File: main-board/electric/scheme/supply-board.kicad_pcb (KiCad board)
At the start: 2 copper layers, 74 x 56 mm, 136 parts, among them K1 CONN_3, P1 PWR-IN, P10 TST, P11 TST, P12 PWR-IN, P13 CONN_4, P14 PWR-IN, P16 TST, P2 PWR-IN, P3 CONN_4, P4 cross board conn, P5 PWR-IN, P6 TST, P7 TST, P8 TST, P9 CONN_3X2, Q1 BC847, Q10 MOS_N, Q11 MOS_P, Q12 MOS_P, Q2 BC847, Q3 BC847, Q4 MOS_P, Q5 BC847, Q6 BC857, Q7 BC847, Q8 BC857, Q9 BC847, U1 NCP3063, U2 L293, U3 MINI-USB-B, X1 8MHz

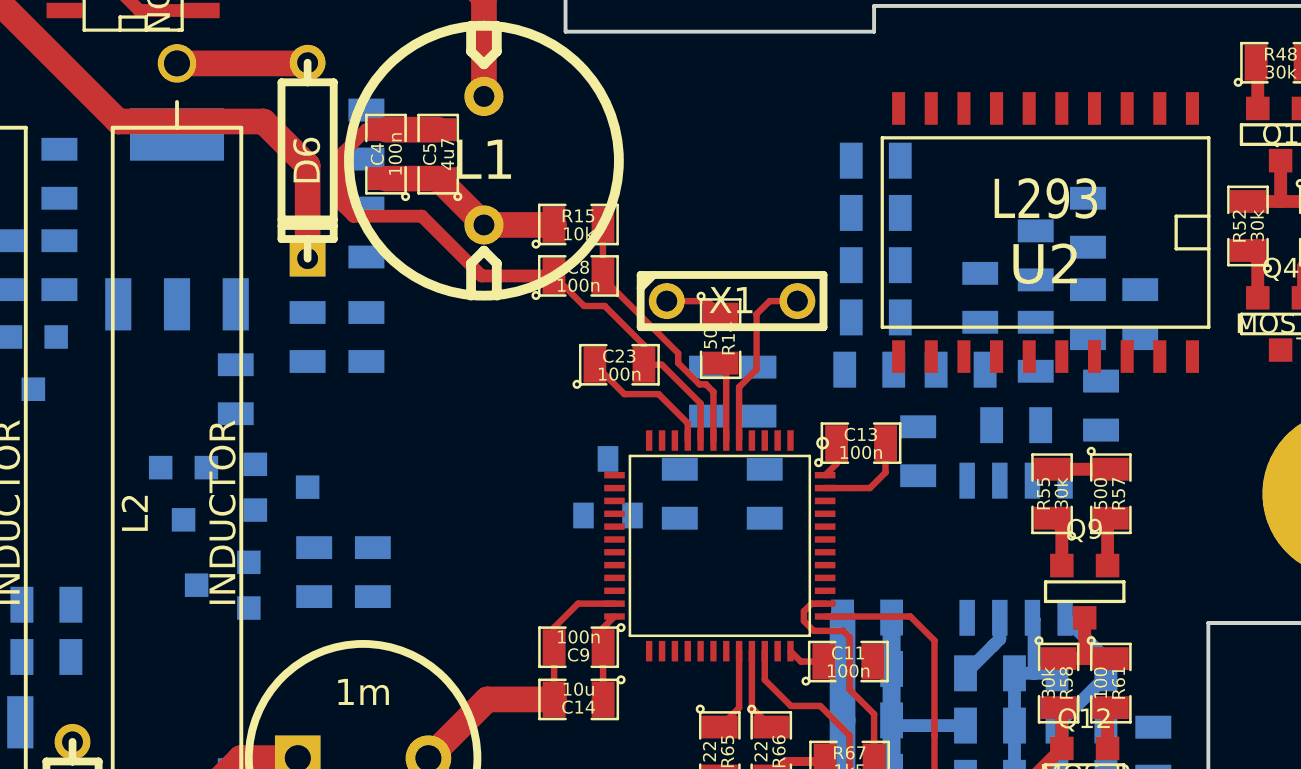
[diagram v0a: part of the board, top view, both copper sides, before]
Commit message: Routing...
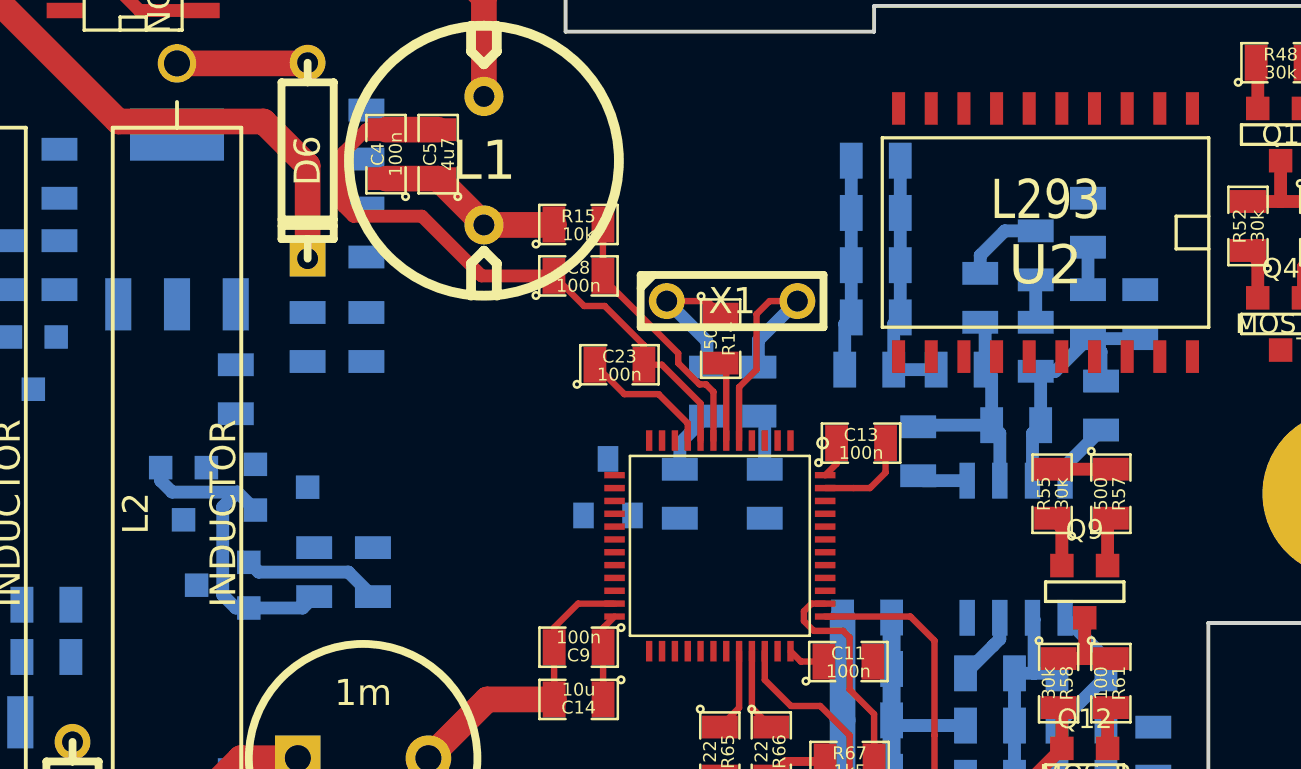
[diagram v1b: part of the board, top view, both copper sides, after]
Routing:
- net N-000008: track 0.00 -> 12.9 mm
- net /in1+: track 0.00 -> 10.9 mm
- net GND: track 157.3 -> 167.8 mm
- net /buck+: track 0.00 -> 9.88 mm
- net /in1-: track 0.00 -> 9.36 mm
- net +6V: track 103.6 -> 111.8 mm
- net N-0000014: track 0.00 -> 5.38 mm
- net N-0000020: track 2.31 -> 5.52 mm
- net N-0000019: track 7.00 -> 10.2 mm
- net /buck-current: track 0.00 -> 1.98 mm
- net N-0000059: track 0.00 -> 1.65 mm
- net N-0000058: track 0.00 -> 1.65 mm
